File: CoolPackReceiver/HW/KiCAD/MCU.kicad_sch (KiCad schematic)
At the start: 23 parts, among them J1 USB_C_Receptacle_USB2.0_16P, U2 STM32U595RJTxQ, Y1 16 MHz

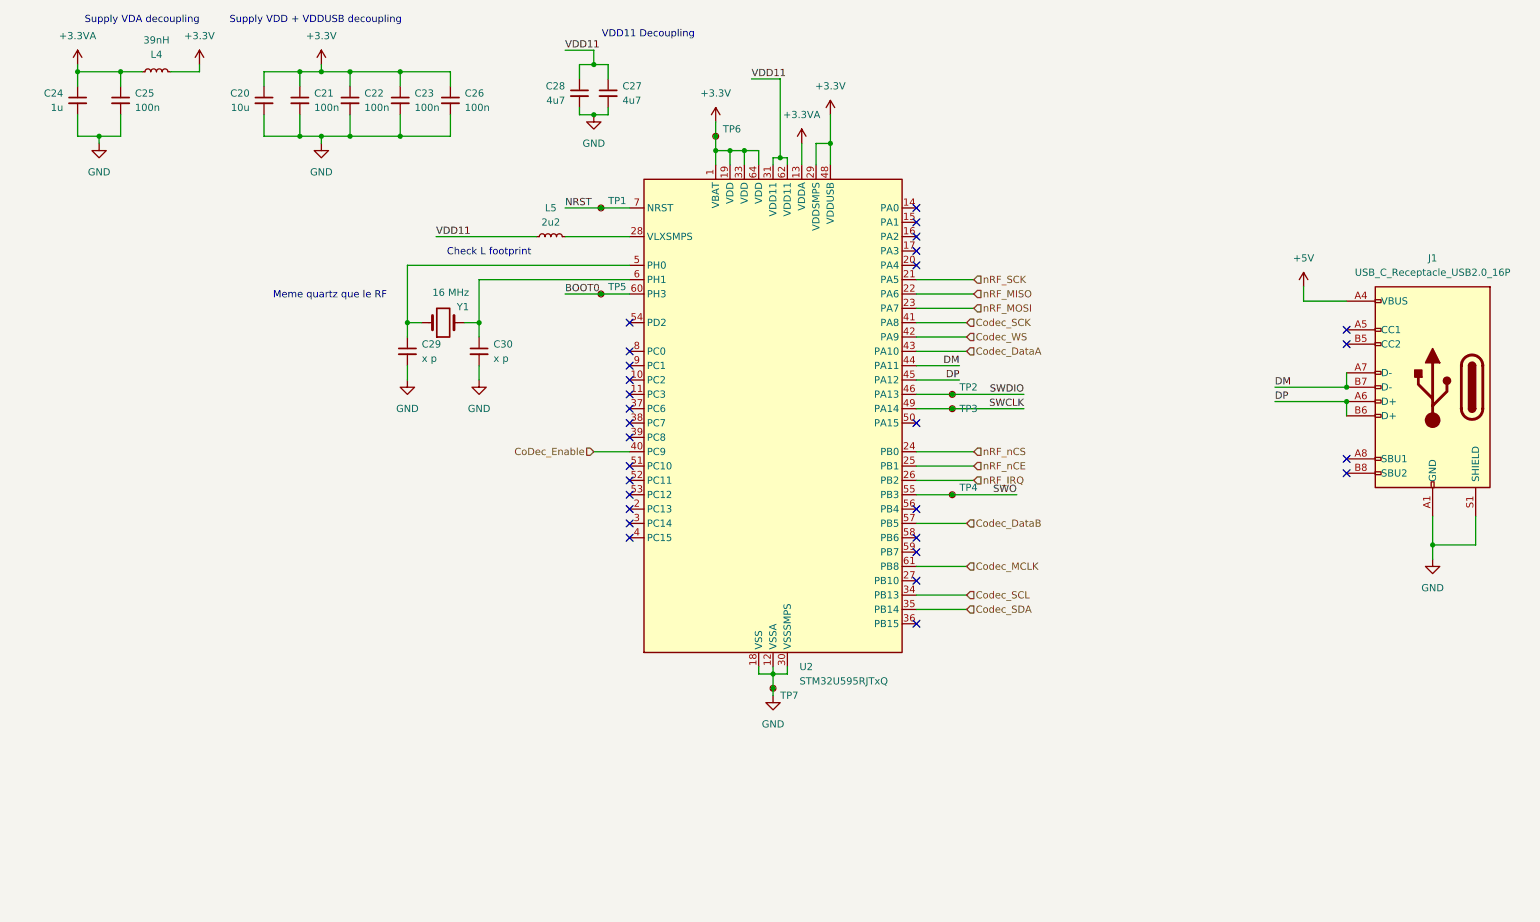
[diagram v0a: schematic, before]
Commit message: CoolPack : Power chain OK
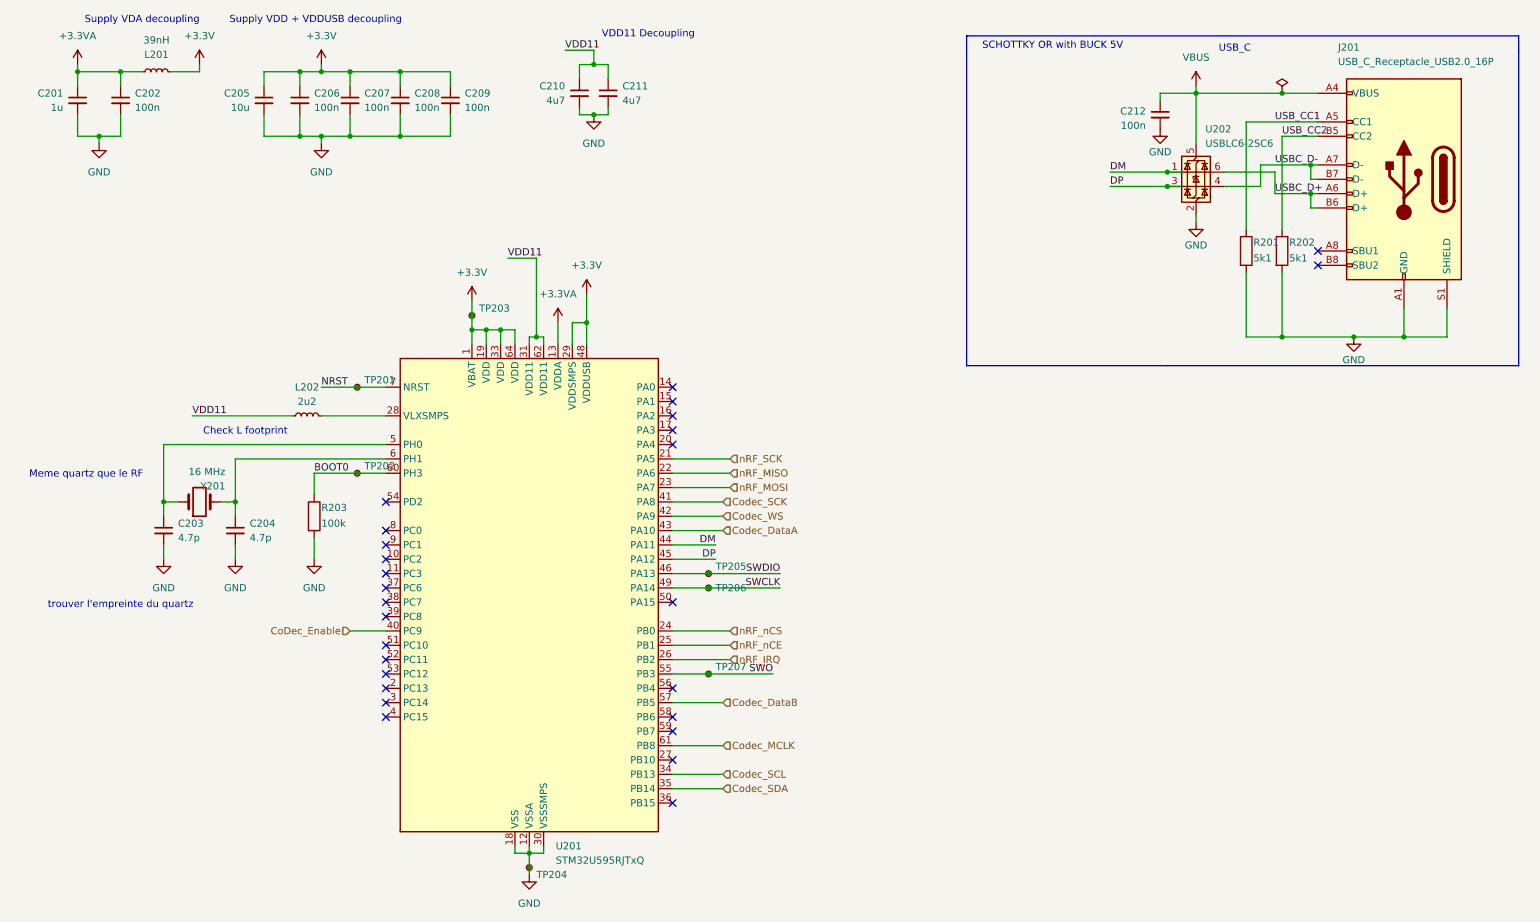
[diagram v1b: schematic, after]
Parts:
- removed C29, C30: x p, Capacitor_SMD:C_0402_1005Metric, symbol Device:C_Small
- removed J1: USB_C_Receptacle_USB2.0_16P, symbol Connector:USB_C_Receptacle_USB2.0_16P
- added C203, C204: 4.7p, Capacitor_SMD:C_0402_1005Metric, symbol Device:C_Small
- added C212: 100n, Capacitor_SMD:C_0402_1005Metric, symbol Device:C_Small
- added J201: USB_C_Receptacle_USB2.0_16P, Connector_USB:USB_C_Receptacle_XKB_U262-16XN-4BVC11, symbol Connector:USB_C_Receptacle_USB2.0_16P
- added R201, R202: 5k1, Resistor_SMD:R_0402_1005Metric, symbol Device:R
- added R203: 100k, Resistor_SMD:R_0402_1005Metric, symbol Device:R
- added U202: USBLC6-2SC6, Package_TO_SOT_SMD:SOT-23-6, symbol Power_Protection:USBLC6-2SC6
- renumbered C24 to C201, C25 to C202, C20 to C205, C21 to C206, C22 to C207, C23 to C208, C26 to C209, C28 to C210, C27 to C211, L4 to L201, L5 to L202, TP1 to TP201, TP5 to TP202, TP6 to TP203, TP7 to TP204, TP2 to TP205, TP3 to TP206, TP4 to TP207, U2 to U201, Y1 to Y201
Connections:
- net BOOT0: now also R203.1
- net DM: now also U202.1 (I/O1)
- net DP: now also U202.3 (I/O2)
- net GND: now also C203.2, C204.2, C212.2, J201.A1 (GND), J201.A12 (GND), J201.B1 (GND), J201.B12 (GND), J201.S1 (SHIELD), R201.2, R202.2, R203.2, U202.2 (GND)
- net at U201.5 (PH0), Y201.1: now also C203.1
- net at U201.6 (PH1), Y201.2: now also C204.1
- new net USBC_D+: J201.A6 (D+), J201.B6 (D+), U202.6 (I/O1)
- new net USBC_D-: J201.A7 (D-), J201.B7 (D-), U202.4 (I/O2)
- new net USB_CC1: J201.A5 (CC1), R201.1
- new net USB_CC2: J201.B5 (CC2), R202.1
- new net VBUS: C212.1, J201.A4 (VBUS), J201.A9 (VBUS), J201.B4 (VBUS), J201.B9 (VBUS), U202.5 (VBUS)
- no-connect marks 29 -> 27
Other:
- note added: "SCHOTTKY OR with BUCK 5V"
- note added: "USB_C"
- note added: "trouver l'empreinte du quartz"
- moved on the sheet: L202, TP201, TP202, TP203, TP204, TP205, TP206, TP207, U201, Y201

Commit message: CoolPack : rooting wip
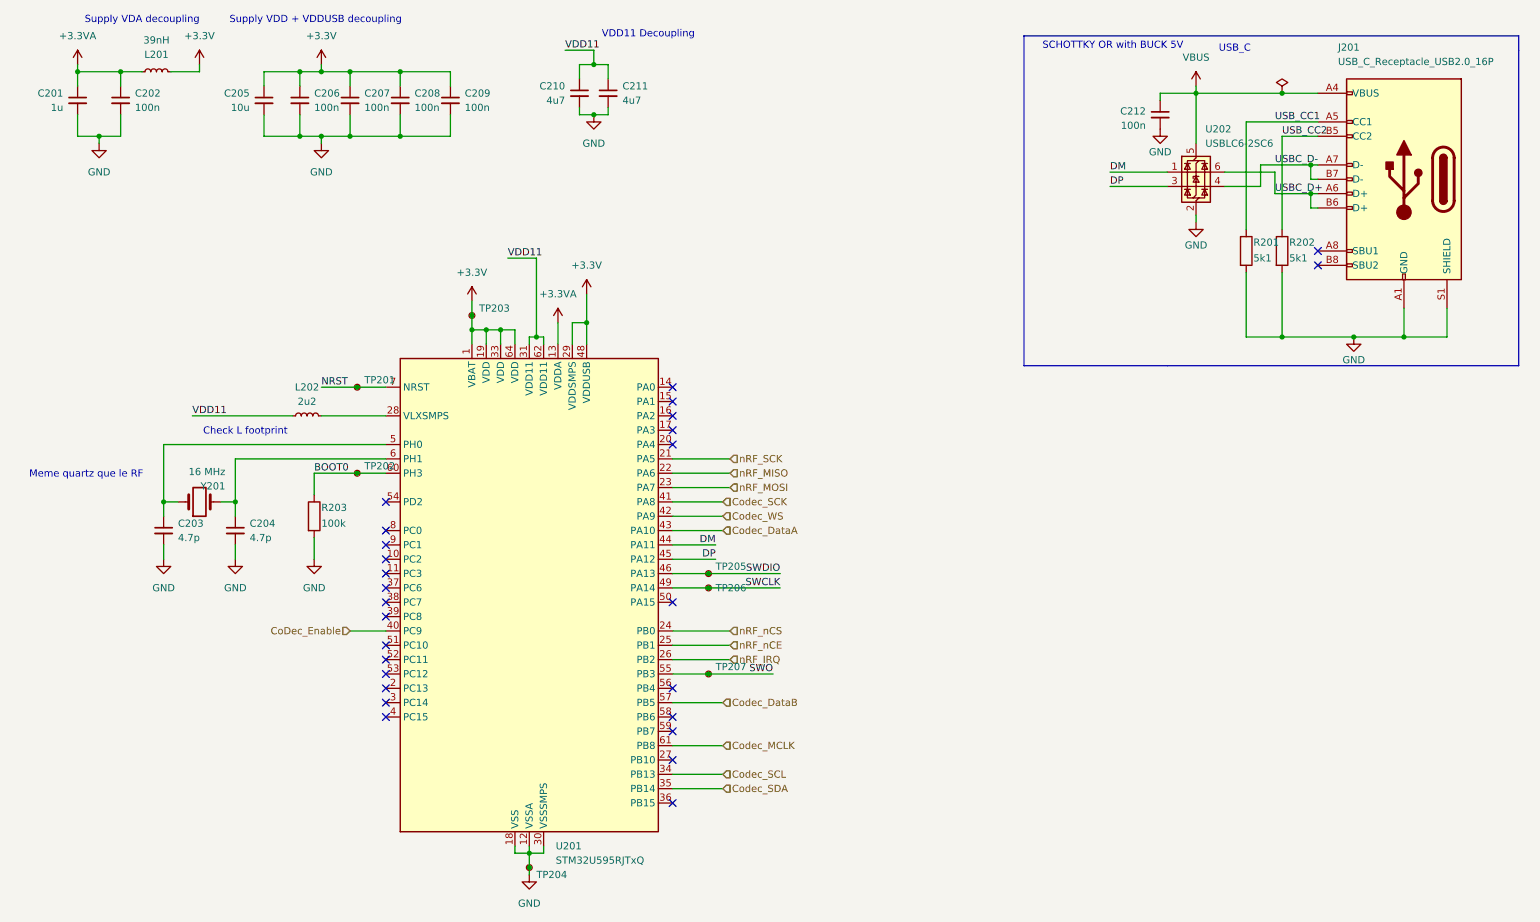
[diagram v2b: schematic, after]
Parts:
- Y201: footprint (none) -> Custom:CX3225FB16000B0FZZH1
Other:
- note removed: "trouver l'empreinte du quartz"
